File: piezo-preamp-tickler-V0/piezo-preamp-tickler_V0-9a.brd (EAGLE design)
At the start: 66.4 x 41.2 mm, 23 parts, among them IC1 TLC272, Q4 2N5484

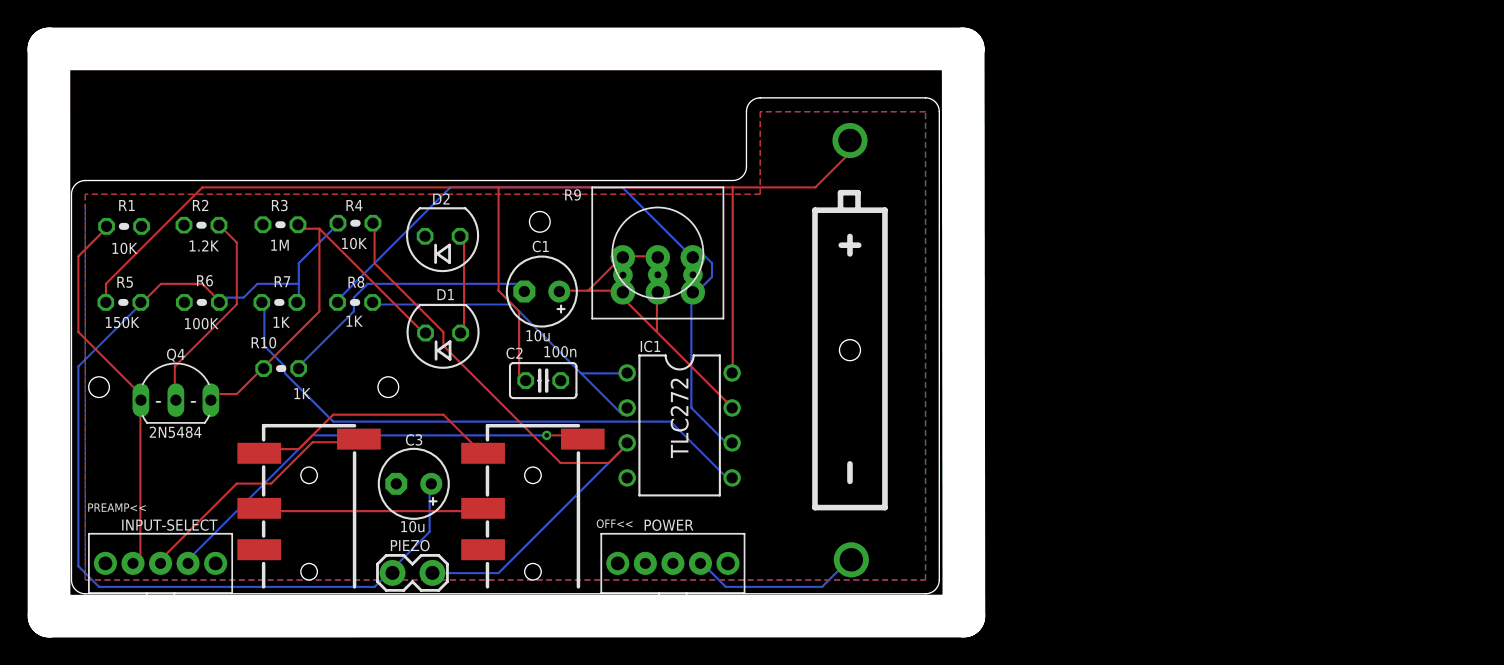
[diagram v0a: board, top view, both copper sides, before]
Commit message: new tickler board
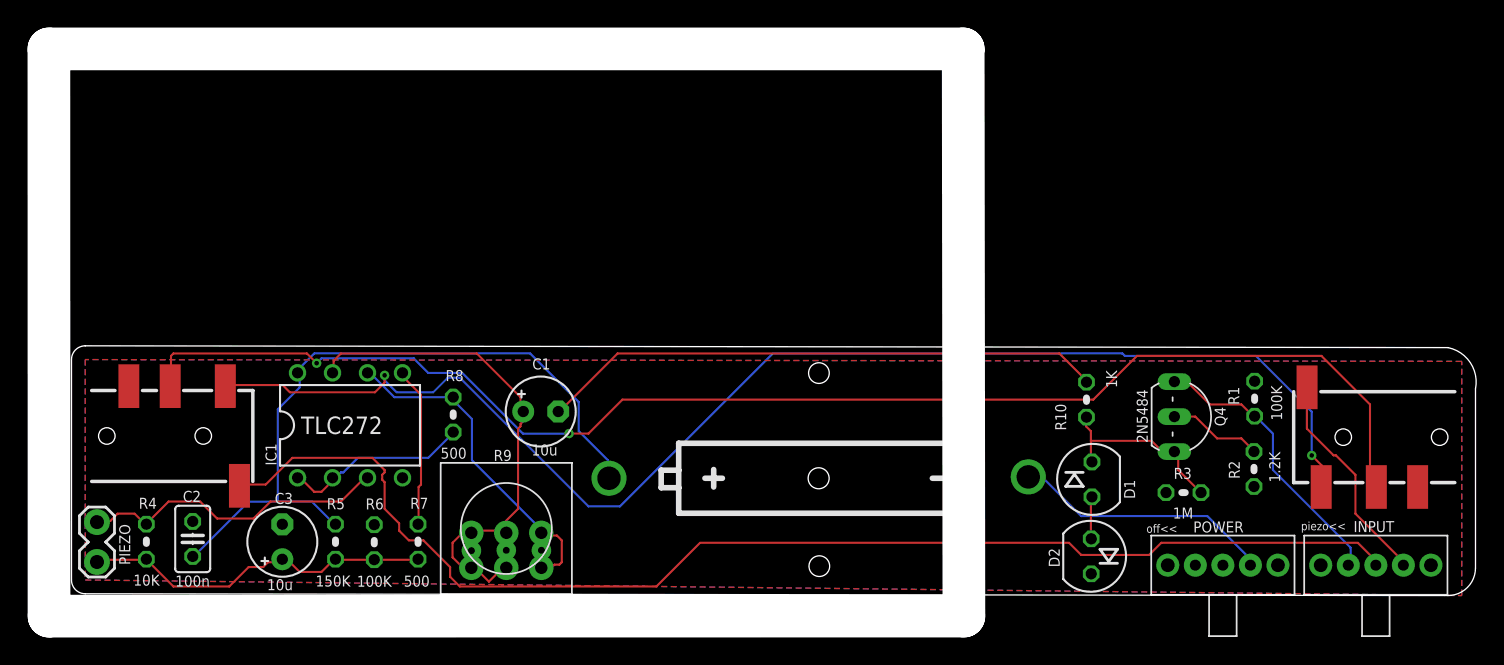
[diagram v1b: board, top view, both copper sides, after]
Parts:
- removed INPUT-SELECT: (no value), Daniel:SPDT-SWITCH
- added INPUT: (no value), Daniel:SPDT-SWITCH
- R1: value 10K -> 100K
- R7, R8: value 1K -> 500
- moved R1 83.0 mm to (85.9, 14.2), turned to 270 degrees
- moved R2 78.4 mm to (85.8, 9.05), turned to 90 degrees
- moved Q4 72.5 mm to (80.1, 12.9), turned to 270 degrees
- moved R3 68.4 mm to (80.7, 7.34)
- moved TO-HEADSET 68.4 mm to (100.9, 11.4), turned to 180 degrees
- moved R10 58.5 mm to (73.7, 14.1), turned to 90 degrees
- moved D2 52.5 mm to (74.0, 2.72), turned to 90 degrees
- moved D1 48.3 mm to (74.1, 8.30), turned to 270 degrees
- moved ON/OFF 39.9 mm to (79.6, 2.08)
- moved C2 27.9 mm to (8.80, 3.98), turned to 270 degrees
- moved R4 27.7 mm to (5.43, 3.78), turned to 270 degrees
- moved PIEZO 24.4 mm to (1.85, 5.03), turned to 270 degrees
- moved IC1 23.9 mm to (20.2, 12.2), turned to 0 degrees
- moved R5 23.2 mm to (19.2, 3.78), turned to 90 degrees
- moved R9 22.8 mm to (31.6, 4.74)
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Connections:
- net N$12: now also INPUT.3; no longer INPUT-SELECT.3
- net TO-PHONE: now also INPUT.2; no longer INPUT-SELECT.2
- net `DEL: now also INPUT.1; no longer INPUT-SELECT.1
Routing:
- net N$15: track 16.4 -> 102.1 mm, vias 0 -> 2
- net N$13: track 18.5 -> 97.1 mm, vias 0 -> 2
- net TO-PHONE: track 18.3 -> 92.6 mm
- net N$8: track 72.5 -> 25.8 mm
- net V9V: track 89.2 -> 51.9 mm
- net N$5: track 41.4 -> 11.7 mm
- net N$7: track 49.9 -> 24.9 mm
- net N$9: track 46.6 -> 22.6 mm
- net N$11: track 20.1 -> 41.0 mm
- net N$12: track 32.8 -> 16.0 mm, vias 1 -> 0
- net N$10: track 29.2 -> 13.6 mm
- net N$14: track 25.5 -> 13.9 mm
- net N$6: track 25.8 -> 36.9 mm
- net N$3: track 15.1 -> 6.85 mm
- net `DEL: track 27.8 -> 20.7 mm
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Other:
- board size 66.4 x 41.2 mm -> 103.6 x 41.2 mm
- board text added: ">>headset"
- board text added: ">>on"
- board text added: "off<<"
- board text added: "piezo<<"
- board text removed: ">>HEADSET"
- board text removed: ">>ON"
- board text removed: "OFF<<"
- board text removed: "PREAMP<<"

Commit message: changes to TeensyLC midi
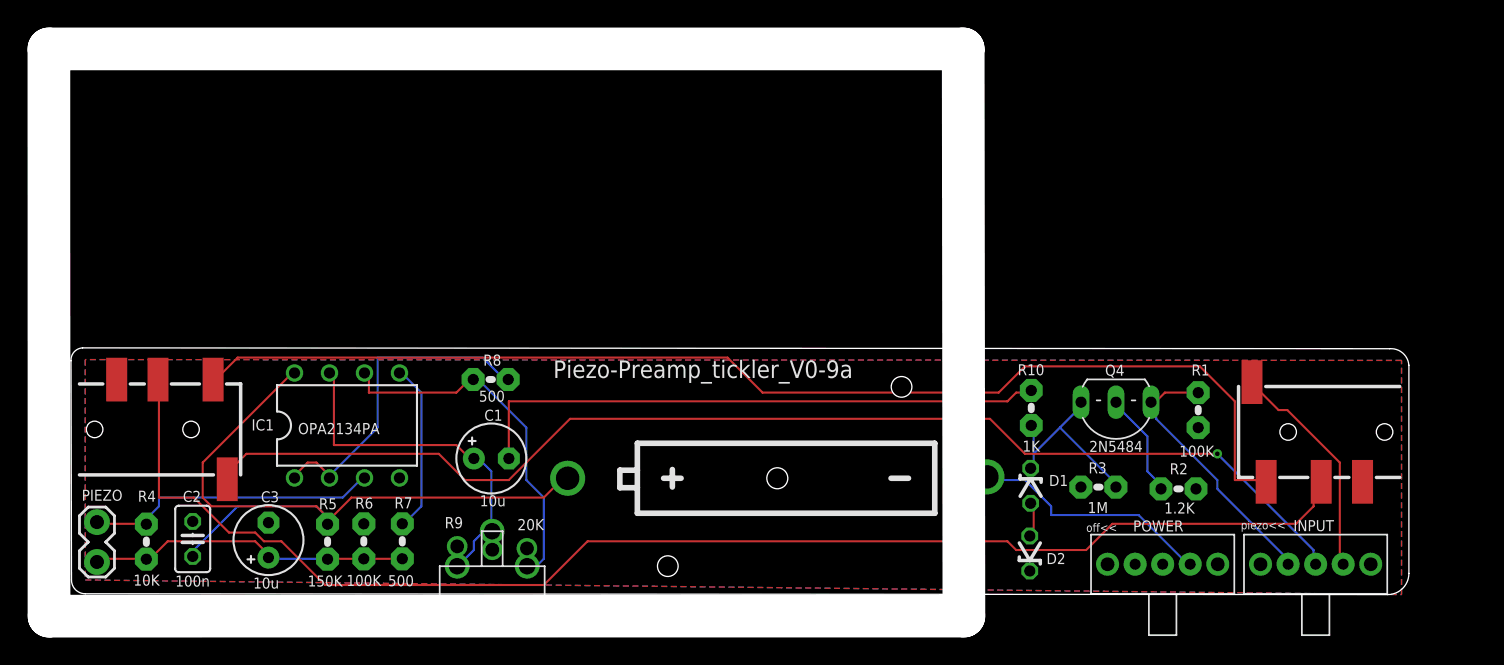
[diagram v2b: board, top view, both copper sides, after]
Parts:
- D1, D2: device diode:SOT54H -> diode:ZDIO-2.5
- IC1: value TLC272 -> OPA2134PA
- R1, R10, R2, R3, R4, R5, R6, R7, R8: device resistor:0204V -> CMU-ArtFab:0204V
- R9: value (none) -> 20K; device Daniel:TRIM-3386 -> CMU-ArtFab:BOURNS-TRIMPOT-3309W1
- moved R3 6.19 mm to (74.5, 7.75)
- moved R2 5.67 mm to (80.4, 7.62), turned to 180 degrees
- moved C1 4.95 mm to (30.5, 9.82)
- moved R9 4.50 mm to (28.0, 2.00)
- moved D1 4.47 mm to (69.6, 7.84)
- moved D2 4.46 mm to (69.6, 2.92)
- moved INPUT 4.37 mm to (86.3, 2.15)
- moved ON/OFF 4.37 mm to (75.2, 2.15)
- moved Q4 4.36 mm to (75.8, 13.9), turned to 180 degrees
- moved R1 4.18 mm to (81.8, 13.3), turned to 90 degrees
- moved R10 4.05 mm to (69.7, 13.5)
- moved TO-HEADSET 4.02 mm to (96.9, 11.7)
- moved R8 3.73 mm to (30.4, 15.6), turned to 180 degrees
- moved BAT1 3.00 mm to (51.2, 8.38)
- moved R7 1.15 mm to (24.0, 3.81)
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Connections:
- net N$6: now also R9.P$1, R9.P$2; no longer R9.1, R9.2, R9.4, R9.5
- net N$7: now also R9.P$3; no longer R9.3, R9.6
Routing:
- net N$13: track 97.1 -> 85.7 mm, vias 2 -> 0
- net N$6: track 36.9 -> 26.8 mm
- net N$14: track 13.9 -> 23.8 mm
- net TO-PHONE: track 92.6 -> 87.5 mm, vias 0 -> 1
- net V9V: track 51.9 -> 54.4 mm
- net N$8: track 25.8 -> 23.5 mm
- net N$15: track 102.1 -> 99.9 mm, vias 2 -> 0
- net N$7: track 24.9 -> 26.8 mm
- net N$2: track 19.1 -> 17.7 mm
- net N$11: track 41.0 -> 42.4 mm
- net `DEL: track 20.7 -> 19.5 mm
- net N$9: track 22.6 -> 21.6 mm
- net N$3: track 6.85 -> 7.81 mm
- net N$10: track 13.6 -> 14.3 mm
- net N$5: track 11.7 -> 12.3 mm
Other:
- board size 103.6 x 41.2 mm -> 98.7 x 41.2 mm
- board text added: "Piezo-Preamp_tickler_V0-9a"
